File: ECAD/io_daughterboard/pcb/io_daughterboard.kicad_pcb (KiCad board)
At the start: 2 copper layers, 120 x 66 mm, 90 parts, among them CON1 BARREL_JACK, J1 XF2L-0625-1A, J2 4-1734839-0, P1 CONN_02X32, P10 Slave 5B, P11 Slave 1C, P12 Slave 3C, P13 Slave 4C, P14 Slave 5C, P15 Slave 1D, P16 Slave 3D, P17 Slave 4D, P18 Slave 5D, P2 CONN_02X32, P3 Slave 1A, P4 Slave 3A, P5 Slave 4A, P6 Slave 5A, P7 Slave 1B, P8 Slave 3B, P9 Slave 4B, U1 FAN5333BSX, U10 SN74LV1T34DCKR, U11 SN74LV1T34DCKR, U2 SPX3819M5-L-3-3, U3 74HC244, U4 74HC244, U5 74HC244, U6 STMPE811QTR, U7 74HC244, U8 74HC244, U9 74HC244

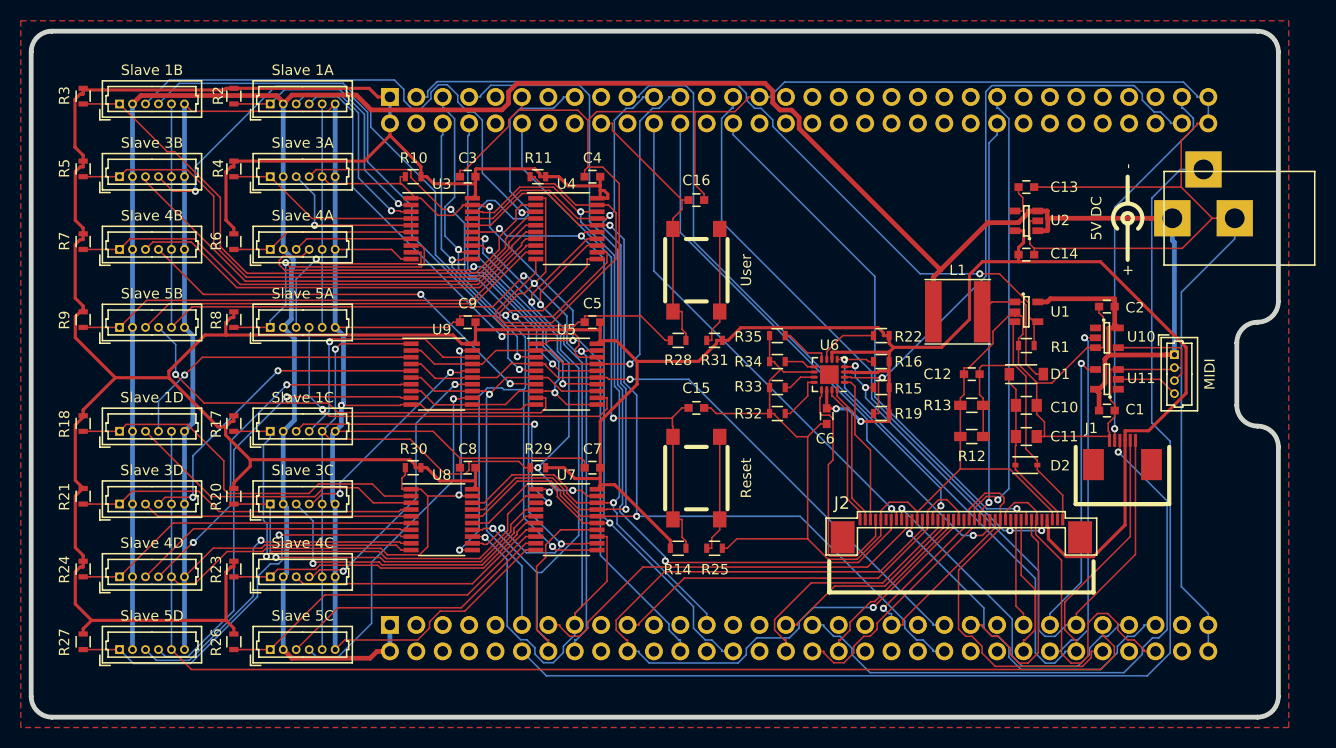
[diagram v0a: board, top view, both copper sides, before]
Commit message: Removed all traces.
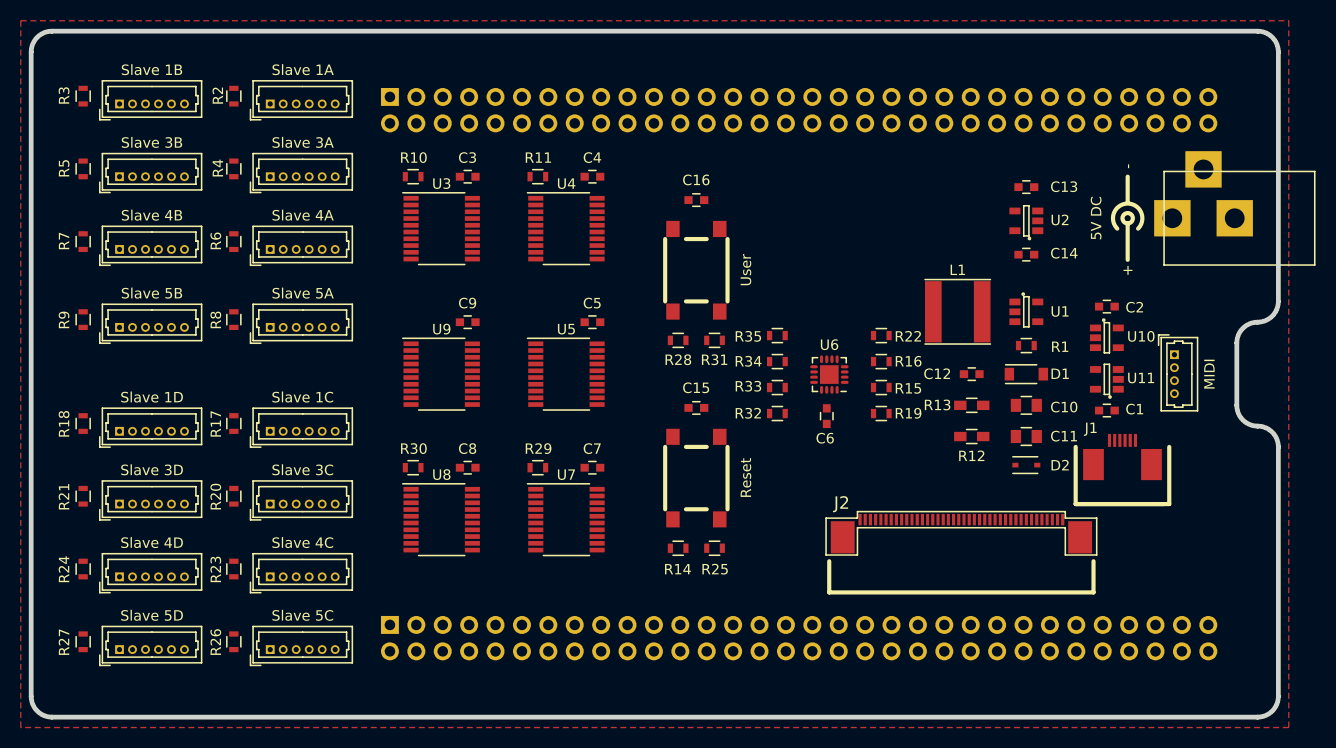
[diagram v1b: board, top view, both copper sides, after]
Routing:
- net GND: track 614.9 -> 0.00 mm, vias 1 -> 0
- net +3V3: track 428.1 -> 0.00 mm, vias 2 -> 0
- net +5V: track 281.8 -> 0.00 mm
- net /PC8: track 173.0 -> 0.00 mm, vias 2 -> 0
- net /PE3: track 141.4 -> 0.00 mm, vias 3 -> 0
- net /PC3: track 122.5 -> 0.00 mm, vias 4 -> 0
- net /PC13: track 114.9 -> 0.00 mm
- net /PC11: track 99.2 -> 0.00 mm, vias 2 -> 0
- net /PB7: track 95.9 -> 0.00 mm, vias 2 -> 0
- net /PF7: track 85.0 -> 0.00 mm, vias 4 -> 0
- net /LCD_DE: track 84.6 -> 0.00 mm, vias 1 -> 0
- net /PE2: track 82.6 -> 0.00 mm, vias 3 -> 0
- net /PE5: track 81.3 -> 0.00 mm, vias 3 -> 0
- net /PF8: track 77.8 -> 0.00 mm, vias 4 -> 0
- net /PA5: track 76.8 -> 0.00 mm, vias 2 -> 0
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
